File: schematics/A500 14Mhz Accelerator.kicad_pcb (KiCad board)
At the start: 2 copper layers, 120.6 x 54.6 mm, 17 parts, among them J1 Speed Selector, U1 68000 Boardside, U10 74HC74, U2 68HC000 Socket, U3 74HC86, U4 74HC74, U5 74LS27, U6 74LS112, U7 74HC04, U8 74LS157, U9 74LS157

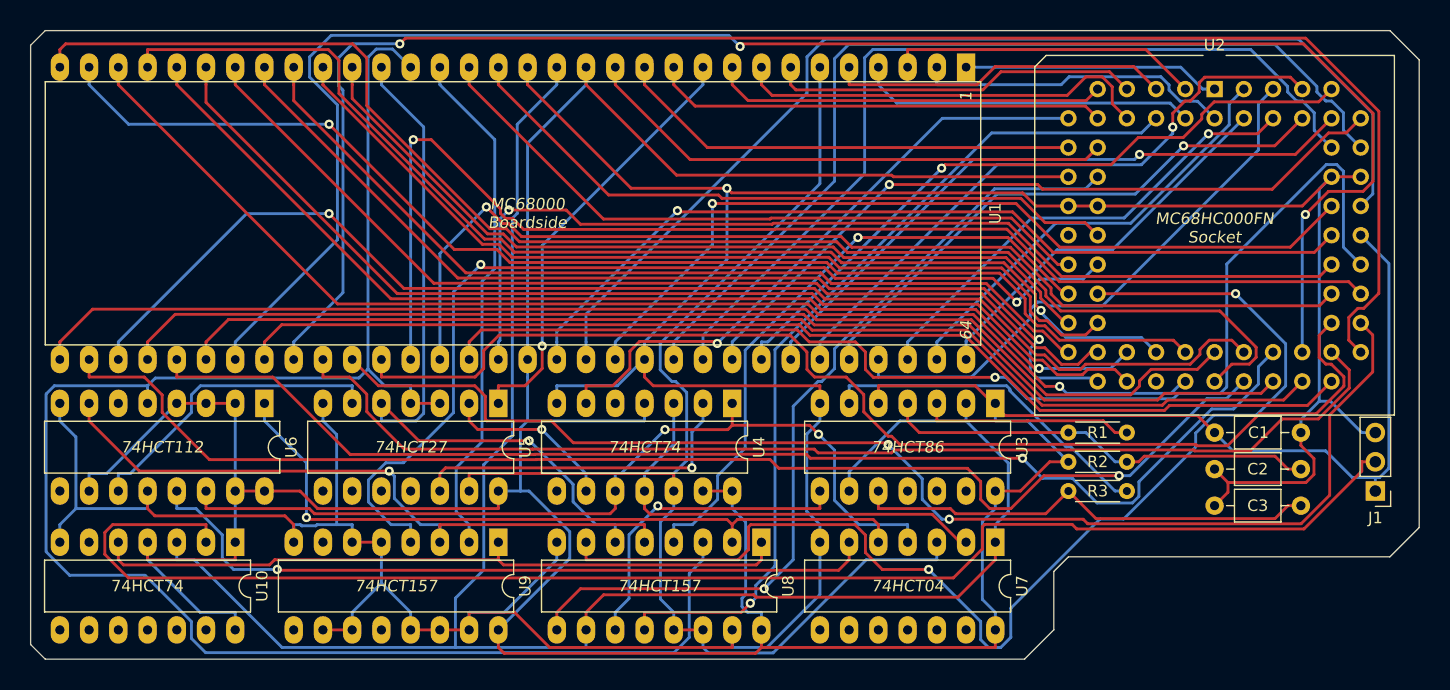
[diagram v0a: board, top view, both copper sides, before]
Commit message: Add files via upload
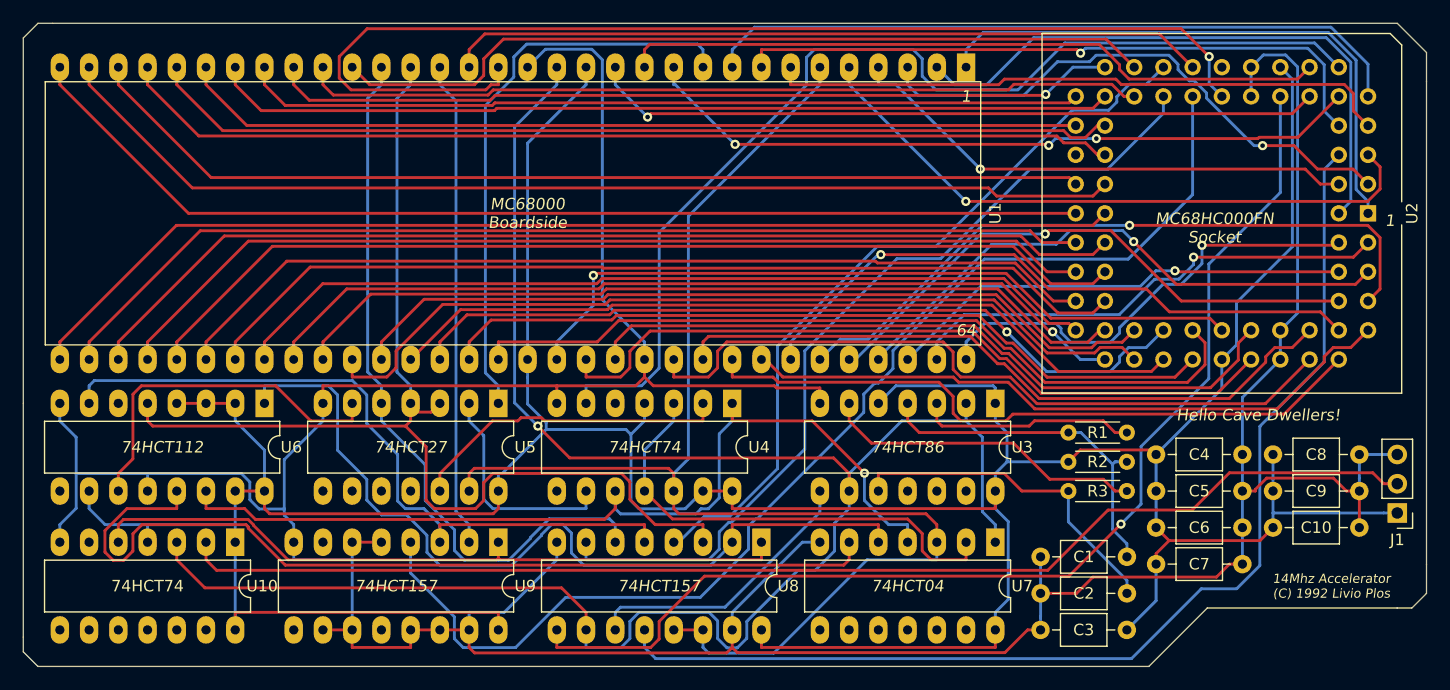
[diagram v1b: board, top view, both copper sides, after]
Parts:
- added C10: 0.1uF, Capacitor_THT:C_Axial_L3.8mm_D2.6mm_P7.50mm_Horizontal, F.Cu at (192.4, 130.2)
- added C4: 0.1uF, Capacitor_THT:C_Axial_L3.8mm_D2.6mm_P7.50mm_Horizontal, F.Cu at (182.2, 123.8)
- added C5: 0.1uF, Capacitor_THT:C_Axial_L3.8mm_D2.6mm_P7.50mm_Horizontal, F.Cu at (182.2, 127.0)
- added C6: 0.1uF, Capacitor_THT:C_Axial_L3.8mm_D2.6mm_P7.50mm_Horizontal, F.Cu at (182.2, 130.2)
- added C7: 0.1uF, Capacitor_THT:C_Axial_L3.8mm_D2.6mm_P7.50mm_Horizontal, F.Cu at (182.2, 133.3)
- added C8: 0.1uF, Capacitor_THT:C_Axial_L3.8mm_D2.6mm_P7.50mm_Horizontal, F.Cu at (192.4, 123.8)
- added C9: 0.1uF, Capacitor_THT:C_Axial_L3.8mm_D2.6mm_P7.50mm_Horizontal, F.Cu at (192.4, 127.0)
- C1: value 0.1uF -> 22pf
- C3: value 22pf -> 0.1uF
- moved C1 18.6 mm to (172.2, 132.7)
- moved C2 18.6 mm to (172.2, 135.9)
- moved U2 17.2 mm to (200.7, 102.9), turned to 270 degrees
- moved C3 13.2 mm to (179.7, 139.1), turned to 180 degrees
- moved J1 2.69 mm to (203.2, 128.9)
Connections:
- C1 pad 1: /VCC -> /GND
- C1 pad 2: /GND -> Net-(C1-Pad2)
- C2 pad 2: Net-(C2-Pad2) -> /A500 14Mhz Accelerator Sheet 2/CDAC
- C3 pad 1: /GND -> /VCC
- C3 pad 2: /A500 14Mhz Accelerator Sheet 2/CDAC -> /GND
- R1 pad 1: Net-(C2-Pad2) -> Net-(C1-Pad2)
- R2 pad 2: Net-(C2-Pad2) -> Net-(C1-Pad2)
- U3 pad 4: Net-(C2-Pad2) -> Net-(C1-Pad2)
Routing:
- net /CPU_A11: track 152.2 -> 81.9 mm, vias 2 -> 0
- net /CPU_A13: track 144.6 -> 76.8 mm
- net /CPU_E: track 153.9 -> 97.3 mm
- net /CPU_HALT: track 59.0 -> 99.3 mm, vias 0 -> 1
- net /CPU_DTACK14: track 54.1 -> 92.3 mm, vias 1 -> 0
- net Net-(C2-Pad2): track 37.8 -> 0.00 mm
- net /CPU_A17: track 107.3 -> 70.2 mm, vias 1 -> 0
- net /CPU_A19: track 104.9 -> 68.2 mm, vias 1 -> 0
- net /CPU_A15: track 111.1 -> 75.6 mm, vias 2 -> 0
- net /CPU_A16: track 102.6 -> 71.2 mm
- net Net-(C1-Pad2): track 0.00 -> 30.8 mm
- net /CPU_A4: track 124.7 -> 94.4 mm
- net /CPU_A22: track 95.2 -> 65.3 mm
- net /CPU_VPA14: track 104.4 -> 75.1 mm, vias 2 -> 0
- net /CPU_D4: track 22.4 -> 50.8 mm
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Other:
- board size 120.6 x 54.6 mm -> 121.9 x 55.9 mm
- board text added: "1"
- board text added: "14Mhz Accelerator (C) 1992 Livio Plos"
- board text added: "Hello Cave Dwellers!"
